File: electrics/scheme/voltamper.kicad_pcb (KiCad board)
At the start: 2 copper layers, 135 parts, among them K1 swd, K2 servo-1, K3 servo-2, P1 boot, P2 boot, P3 -, P4 +, P5 work, P6 aux, P7 ref, Q1 bc857, Q2 bc847, Q3 bc857, Q4 bc847, Q5 irlml2244, Q6 bc847, Q7 bc847, Q8 bc847, SW1 btn-1, SW2 btn-2, U1 CRYSTAL-4PIN, U10 TDA2030A, U11 INA126, U12 SPARTAN-SIP-9007, U2 CP2102, U3 MICRO-USB-B, U4 MCP1703T-3302E/CB, U5 MCP1703T-3302E/CB, U6 NCP3063, U7 SPARTAN-SIP-9007, U8 NCP3063, U9 SPARTAN-SIP-9007

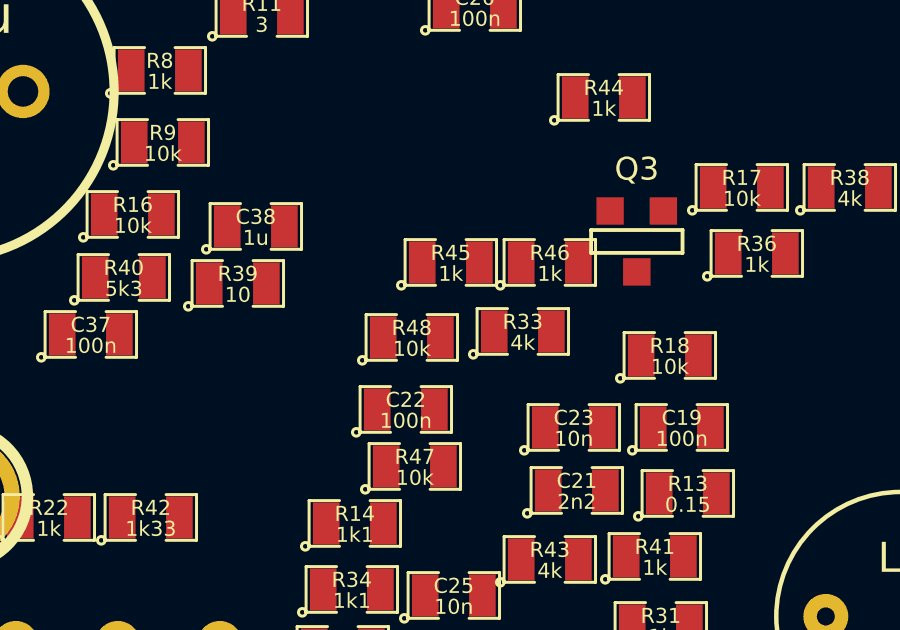
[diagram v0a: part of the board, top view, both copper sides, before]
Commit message: a
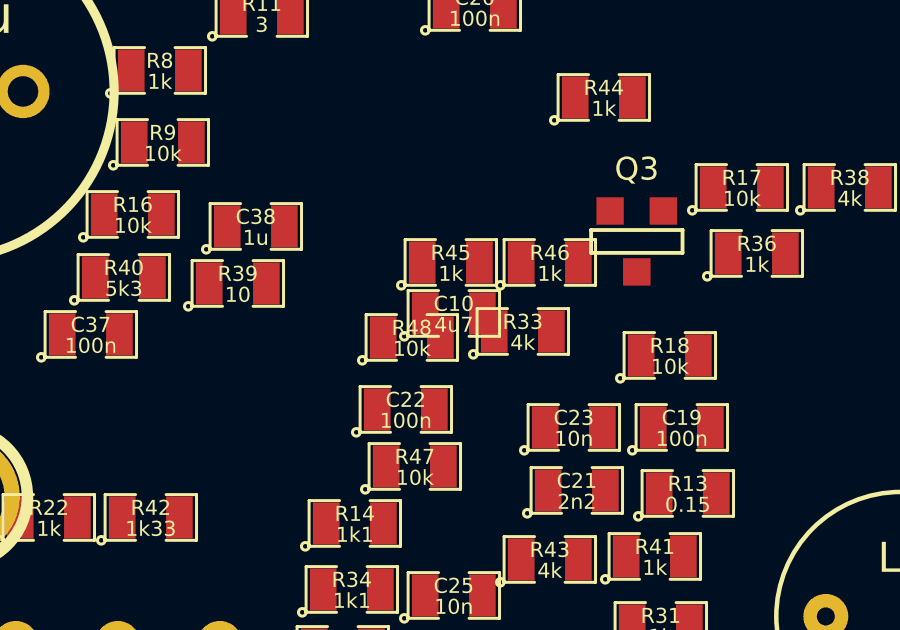
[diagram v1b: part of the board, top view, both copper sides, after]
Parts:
- added C10: 4u7, SM0805, F.Cu at (0.00, 0.00)
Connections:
- U2 pad 10: N-0000094 -> VDD
- U2 pad 13: N-0000094 -> VDD
- U2 pad 14: N-0000094 -> VDD
- U2 pad 15: N-0000094 -> VDD
- U2 pad 16: N-0000094 -> VDD
- U2 pad 17: N-0000094 -> VDD
- U2 pad 18: N-0000094 -> N-0000061
- U2 pad 19: N-0000094 -> VDD
- U2 pad 20: N-0000094 -> VDD
- U2 pad 21: N-0000094 -> VDD
- U2 pad 22: N-0000094 -> VDD
